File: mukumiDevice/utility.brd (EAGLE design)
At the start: 50.9 x 40.6 mm, 11 parts

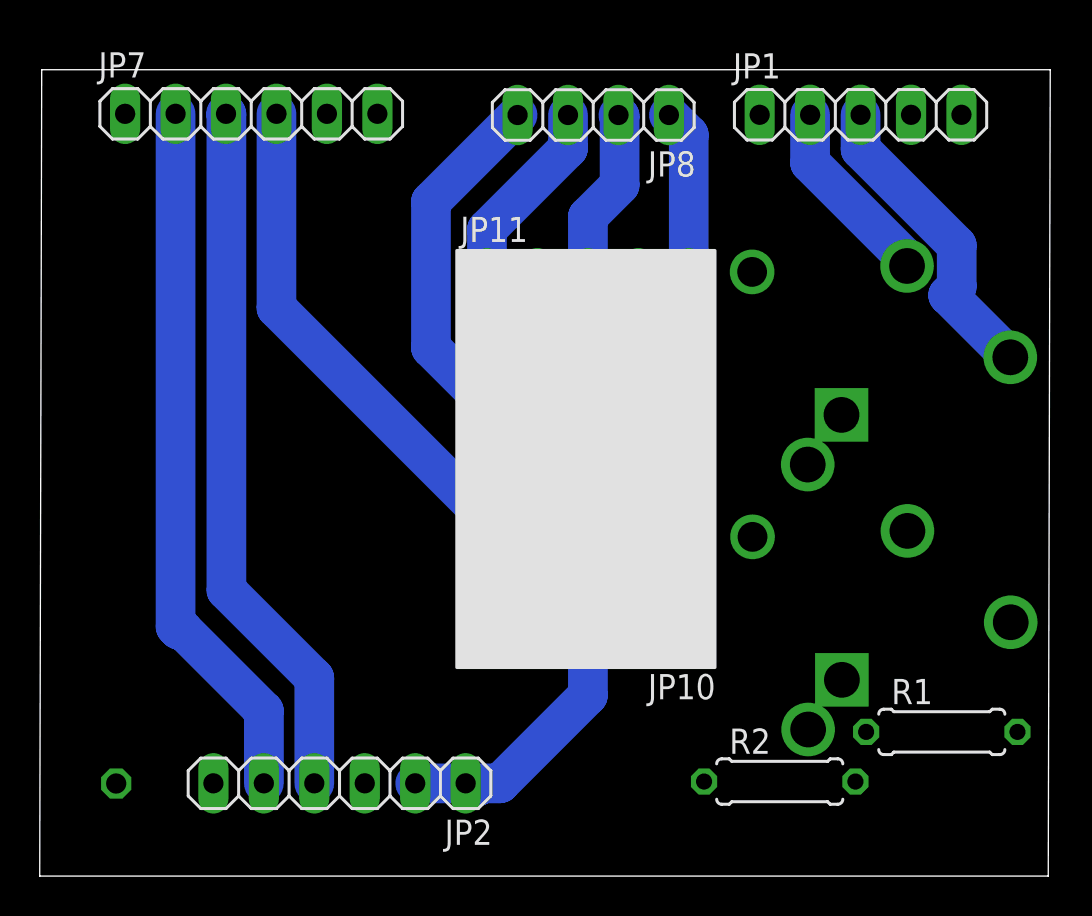
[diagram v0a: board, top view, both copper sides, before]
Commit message: ジャック部の修正
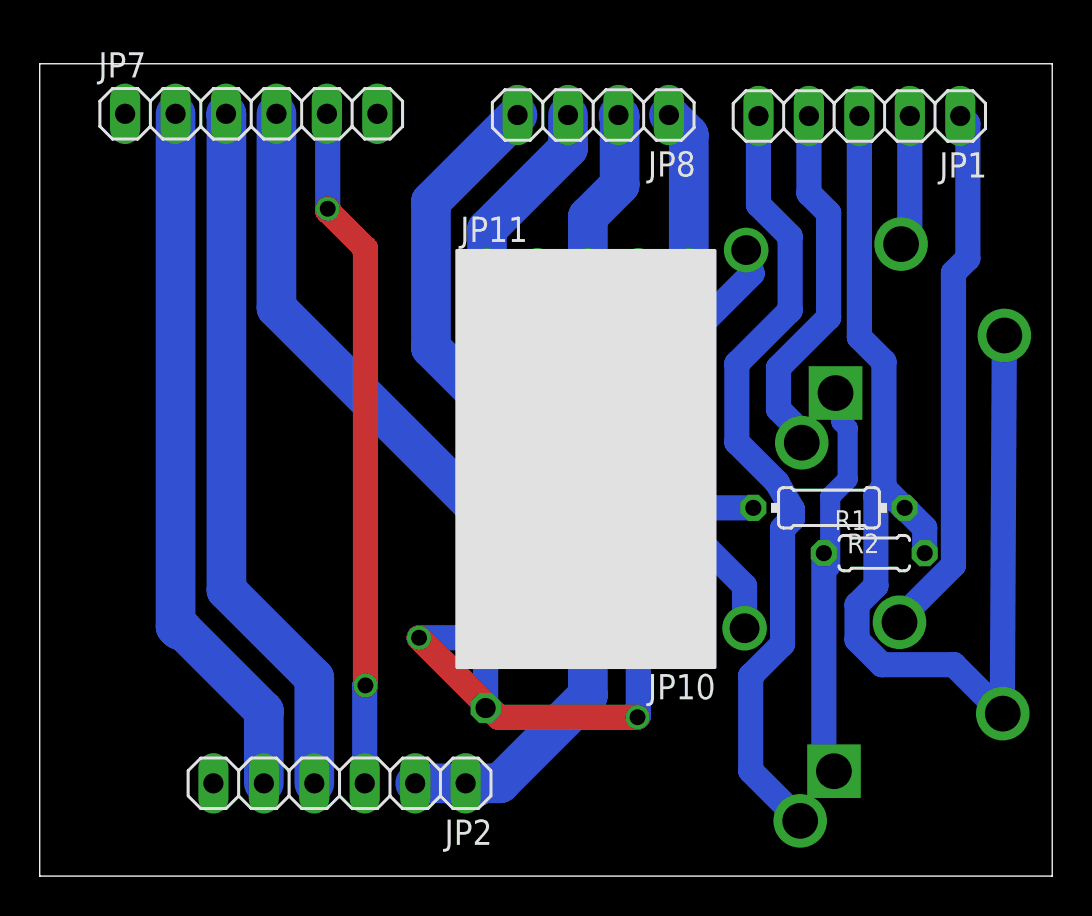
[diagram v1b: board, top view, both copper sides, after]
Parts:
- R1: device rcl:0207/7 -> rcl:0204/5
- R2: device rcl:0207/7 -> rcl:0204/7
- moved JP9 19.0 mm to (22.4, 8.46)
- moved R2 14.0 mm to (39.7, 18.5), turned to 180 degrees
- moved R1 9.62 mm to (42.0, 16.3)
- moved CURRENT_OUT 4.62 mm to (48.5, 8.18)
- moved MESURE_VOL 1.14 mm to (48.6, 27.2)
- moved JP1 0.08 mm to (41.3, 38.3), turned to 180 degrees
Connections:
- net N$1: now also R1.2, R2.1
- net N$4: no longer R1.2, R2.1
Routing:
- net N$1: track 15.7 -> 60.4 mm
- net N$3: track 0.00 -> 40.7 mm
- net VCC: track 0.00 -> 34.5 mm, vias 0 -> 2
- net N$2: track 0.00 -> 27.1 mm
- net N$8: track 0.00 -> 26.0 mm
- net SW: track 0.00 -> 23.7 mm, vias 0 -> 2
- net N$7: track 0.00 -> 21.2 mm
- net N$5: track 0.00 -> 18.7 mm
- net N$4: track 9.63 -> 6.63 mm
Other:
- board size 50.9 x 40.6 mm -> 51 x 40.9 mm
